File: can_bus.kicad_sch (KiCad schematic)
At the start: 1 part, among them U8 MCP2562-E-SN

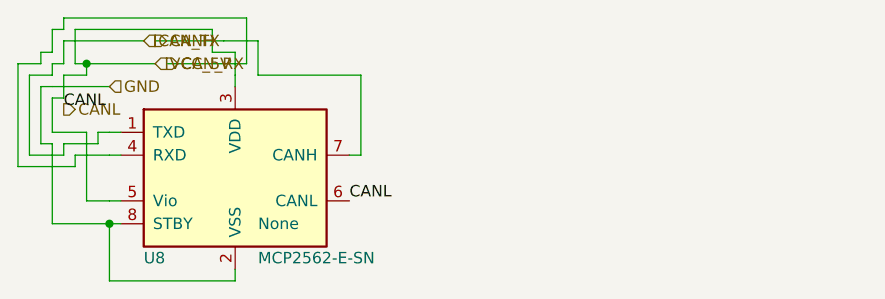
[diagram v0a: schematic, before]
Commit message: refactoring
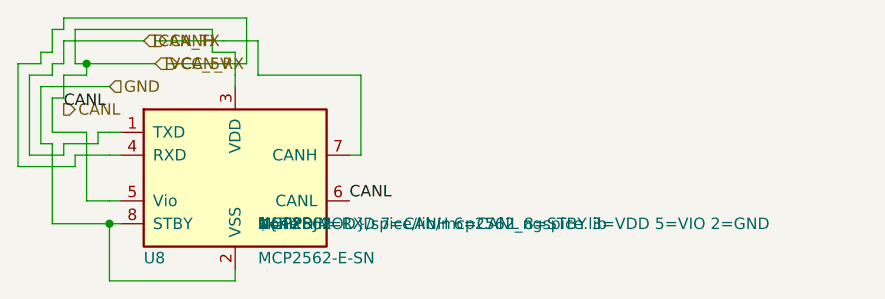
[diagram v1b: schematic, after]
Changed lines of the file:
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@@
+			)
+		)
+		(property "Sim.Device" "X"
+			(at 38.1 29.2099 0)
+			(effects
+				(font
+					(size 1.27 1.27)
+				)
+				(justify left)
+			)
+		)
+		(property "Sim.Name" "MCP2562"
+			(at 38.1 29.2099 0)
+			(effects
+				(font
+					(size 1.27 1.27)
+				)
+				(justify left)
+			)
+		)
+		(property "Sim.Library" "${KIPRJMOD}/spice/lib/mcp2562_ngspice.lib"
+			(at 38.1 29.2099 0)
+			(effects
+				(font
+					(size 1.27 1.27)
+				)
+				(justify left)
+			)
+		)
+		(property "Sim.Pins" "1=TXD 4=RXD 7=CANH 6=CANL 8=STBY 3=VDD 5=VIO 2=GND"
+			(at 38.1 29.2099 0)
+			(effects
+				(font
+					(size 1.27 1.27)
+				)
+				(justify left)
+			)
+		)
+		(property "Sim.Enable" "1"
+			(at 38.1 29.2099 0)
+			(effects
+				(font
+					(size 1.27 1.27)
+				)
+				(justify left)
 			)
 		)
@@
 		(instances
 			(project "climate_control_niva_travel"
-				(path "/165a98f1-2dde-4141-9fdc-c935d39c8cff/07ec9d0b-cd95-49f4-92c1-d02e79bd1c75/"
+				(path "/cc416b40-1361-4232-ac1e-5cd36ef0c0fb/c39f5ba4-c7f2-413a-b1c4-1fa4d87e42a0/"
 					(reference "U0808")
 					(unit 1)
@@
 	(junction
 		(at 19.05 11.43)
-		(diameter 0)
+		(diameter 0.0000)
 		(color 0 0 0 0)
 	)
 	(junction
 		(at 21.59 29.21)
-		(diameter 0)
+		(diameter 0.0000)
 		(color 0 0 0 0)
 	)
